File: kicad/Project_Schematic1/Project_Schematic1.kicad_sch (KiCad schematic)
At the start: 46 parts, among them M1 Flag_Servo, M2 Motor_Left, M3 Motor_Bottom, M4 Motor_Right, Q1 NPN, Q2 NPN, Q3 NPN, U1 74xxx244, U10 MCP6294, U11 MCP6294, U12 SW_CapTouch, U2 PIC32MX170F256B, U3 CD4052, U4 QTR-HD-01A, U5 Left_Drum_LEDs, U6 Bottom_Drum_LEDs, U7 Right_Drum_LEDs, U8 Clock_LEDs, U9 MCP6294

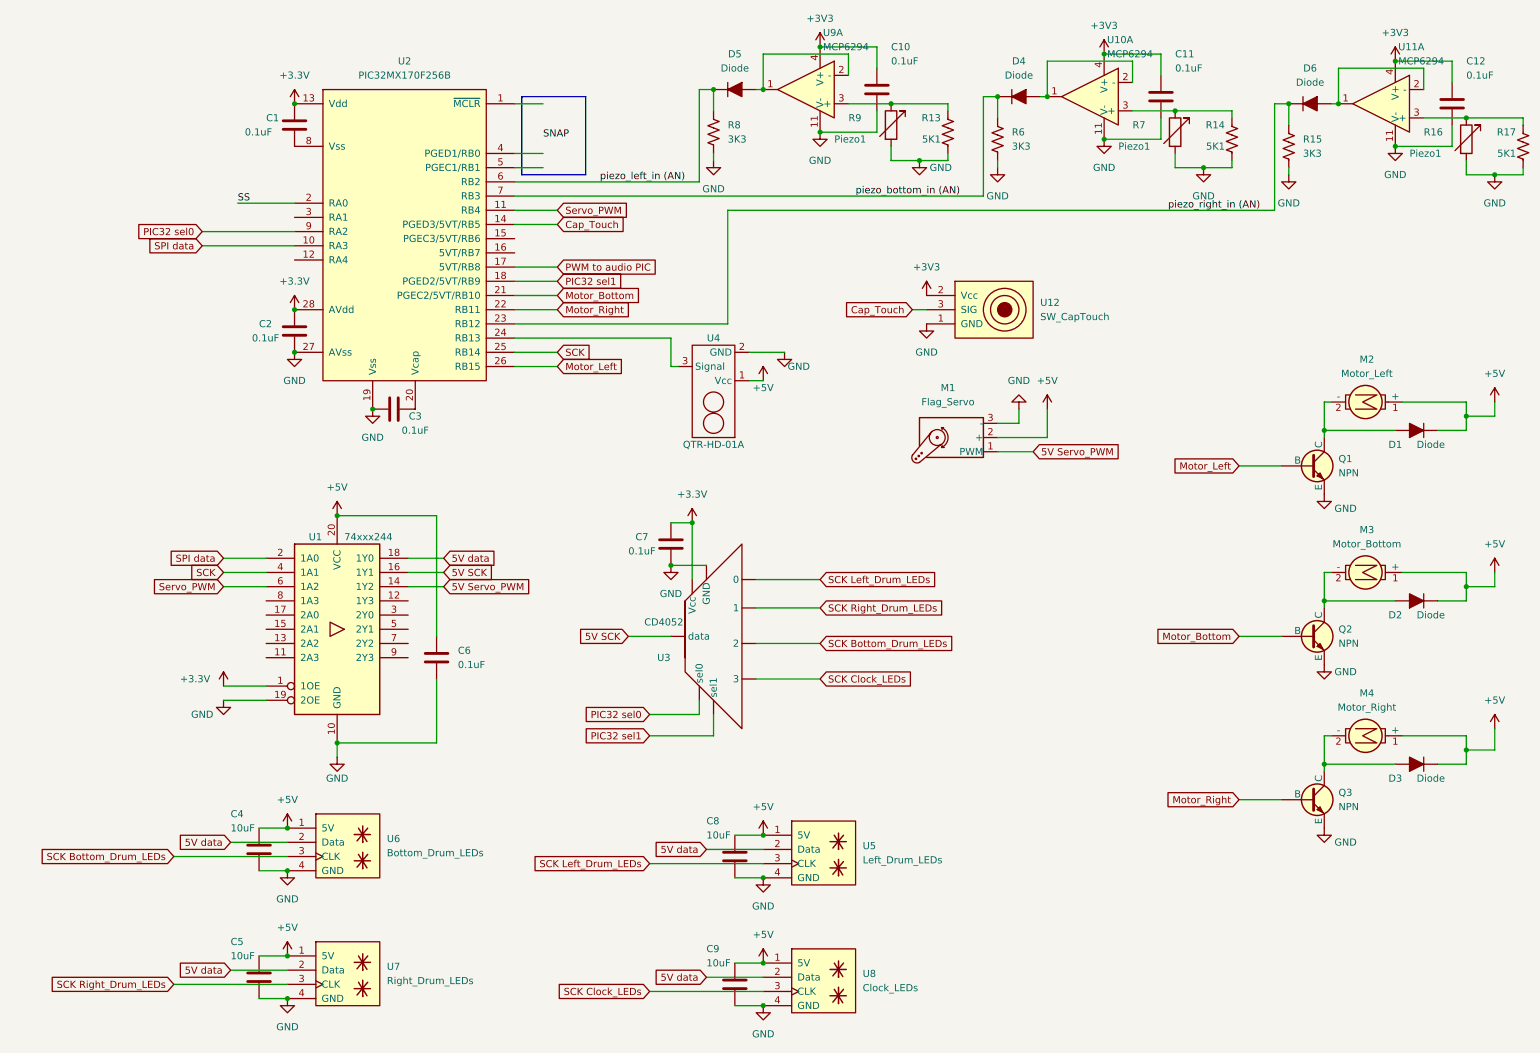
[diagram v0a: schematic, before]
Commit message: Revert to 3d98758
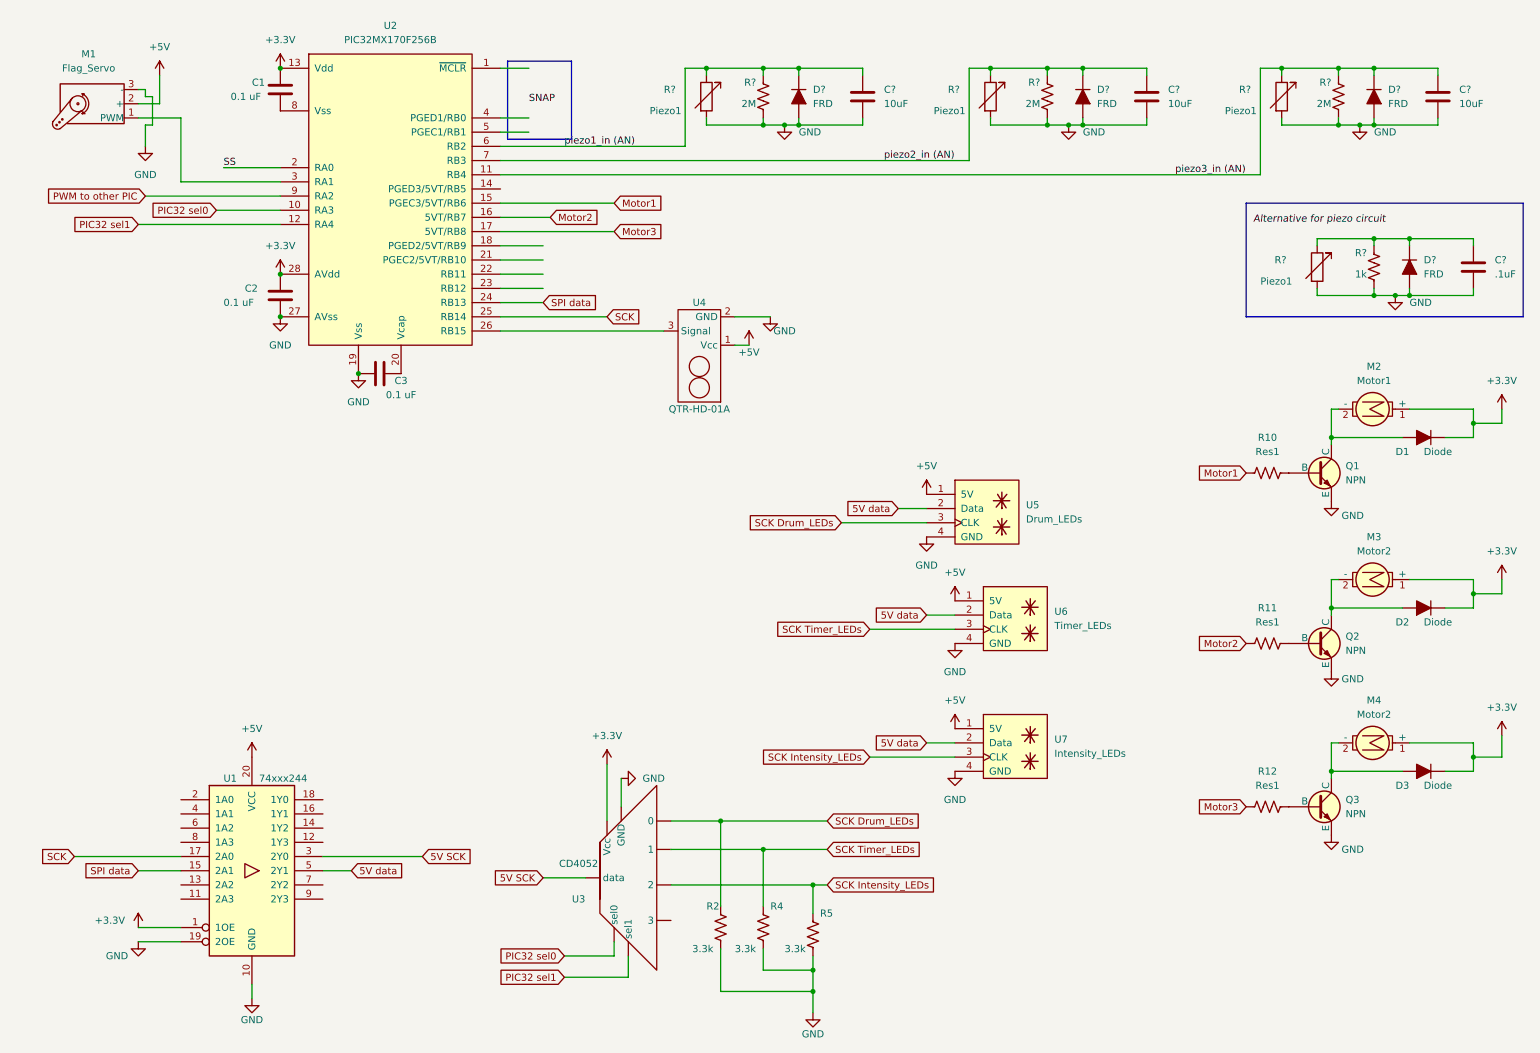
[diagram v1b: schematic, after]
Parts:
- removed C10, C11, C12, C6, C7: 0.1uF, symbol ME218_BaseLib:Cap
- removed C4, C5, C8, C9: 10uF, symbol ME218_BaseLib:Cap
- removed D4, D5, D6: Diode, symbol ME218_BaseLib:Diode
- removed R14, R17: 5K1, symbol ME218_BaseLib:Res1
- removed R15, R6, R8: 3K3, symbol ME218_BaseLib:Res1
- removed R16, R7: Piezo1, symbol ME218_BaseLib:Res_Adj2
- removed U10, U11, U9: MCP6294, symbol ME218_BaseLib:MCP6294
- removed U12: SW_CapTouch, symbol ME218_BaseLib:SW_CapTouch
- removed U8: Clock_LEDs, symbol ME218_BaseLib:Dot_Star
- added C?: .1uF, symbol ME218_BaseLib:Cap
- added C? (x3): 10uF, symbol ME218_BaseLib:Cap
- added D? (x4): FRD, symbol ME218_BaseLib:Diode
- added R10, R11, R12: Res1, symbol ME218_BaseLib:Res1
- added R2, R4, R5: 3.3k, symbol ME218_BaseLib:Res1
- added R? (x3): Piezo1, symbol ME218_BaseLib:Res_Adj2
- added R?: 1k, symbol ME218_BaseLib:Res1
- added R? (x2): 2M, symbol ME218_BaseLib:Res1
- C1, C2, C3: value 0.1uF -> 0.1 uF
- M2: value Motor_Left -> Motor1
- M3: value Motor_Bottom -> Motor2
- M4: value Motor_Right -> Motor2
- R?: renamed from R13; value 5K1 -> 2M
- U5: value Left_Drum_LEDs -> Drum_LEDs
- U6: value Bottom_Drum_LEDs -> Timer_LEDs
- U7: value Right_Drum_LEDs -> Intensity_LEDs
- renumbered R9 to R?
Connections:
- net SCK Clock_LEDs is gone; now on net SCK Timer_LEDs: U3. (sel1)
- net piezo_left_in (AN) is gone; now on net piezo1_in (AN): U2.6 (RB2)
- net +3.3V: now also D1.1 (K), D2.1 (K), D3.1 (K), M2.1 (+), M3.1 (+), M4.1 (+)
- net +5V: no longer D1.1 (K), D2.1 (K), D3.1 (K), M2.1 (+), M3.1 (+), M4.1 (+)
- net 5V SCK: now also U1.3 (2Y0); no longer U1.16 (1Y1)
- net 5V data: now also U1.5 (2Y1); no longer U1.18 (1Y0)
- net GND: now also C?.2, C?.2, C?.2, C?.2, D?.2 (A), D?.2 (A), D?.2 (A), D?.2 (A), R2.2, R4.2, R5.2, R?.1, R?.1, R?.1, R?.2, R?.2, R?.2
- net PIC32 sel0: now also U2.10 (RA3); no longer U2.9 (RA2)
- net PIC32 sel1: now also U2.12 (RA4); no longer U2.18 (PGED2/5VT/RB9)
- net SCK: now also U1.17 (2A0); no longer U1.4 (1A1)
- net SPI data: now also U1.15 (2A1), U2.24 (RB13); no longer U1.2 (1A0), U2.10 (RA3)
- net piezo1_in (AN): now reaches R?.1, R?.2
- net piezo1_in (AN): now also C?.1, D?.1 (K)
- net Motor1: now reaches U2.15 (PGEC3/5VT/RB6)
- net Motor1: now also R10.1
- net Motor2: now reaches U2.16 (5VT/RB7)
- net Motor2: now also R11.1
- net at U4.3 (Signal): now also U2.26 (RB15); no longer U2.24 (RB13)
- net at U2.3 (RA1): now also M1.1 (PWM)
- net 5V Servo_PWM: no longer names the net of U1.14 (1Y2)
- net 5V Servo_PWM: no longer M1.1 (PWM)
- net Cap_Touch: no longer names the net of U2.14 (PGED3/5VT/RB5)
- net Motor_Bottom: no longer names the net of U2.21 (PGEC2/5VT/RB10)
- net Motor_Bottom: no longer Q2.1 (B)
- net Motor_Left: no longer names the net of Q1.1 (B)
- net Motor_Left: now also R10.2; no longer U2.26 (RB15)
- net Motor_Right: no longer names the net of U2.22 (RB11)
- net Motor_Right: no longer Q3.1 (B)
- net PWM to audio PIC renamed Motor3
- net Motor3: now also R12.1
- net SCK Bottom_Drum_LEDs renamed SCK Timer_LEDs
- net SCK Timer_LEDs: now also R4.1
- net SCK Left_Drum_LEDs renamed SCK Drum_LEDs
- net SCK Drum_LEDs: now also R2.1
- net SCK Right_Drum_LEDs renamed SCK Intensity_LEDs
- net SCK Intensity_LEDs: now also R5.1
- net Servo_PWM: no longer names the net of U1.6 (1A2)
- net Servo_PWM: no longer U2.11 (RB4)
- net piezo_bottom_in (AN) renamed piezo2_in (AN)
- net piezo2_in (AN): now also C?.1, D?.1 (K), R?.1, R?.2
- net piezo_right_in (AN): no longer names the net of U2.23 (RB12)
- new net: C?.1, D?.1 (K), R?.1, R?.2
- new net: Q3.1 (B), R12.2
- new net: Q2.1 (B), R11.2
- new net PWM to other PIC: U2.9 (RA2)
- new net piezo3_in (AN): C?.1, D?.1 (K), R?.1, R?.2, U2.11 (RB4)
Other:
- moved on the sheet: C1, C2, C3, D1, D2, D3, M1, M2, M3, M4, Q1, Q2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
